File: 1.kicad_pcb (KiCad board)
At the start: 2 copper layers, 85.1 x 46.4 mm, 44 parts, among them J1 Micro_SD_Card, J10 I2C1, J11 I2C2, J12 B3..9A, J2 USB_B_Micro, J3 Conn_Power, J4 SWD, J5 Protected, J6 SPI1, J7 ADC, J8 UART1, J9 SPI2, K1 NRST, K2 WKUP, K3 KPA0, U1 STM32F103C8Tx, U2 AMS1117-3.3, Y1 8MHz, Y2 32.768k

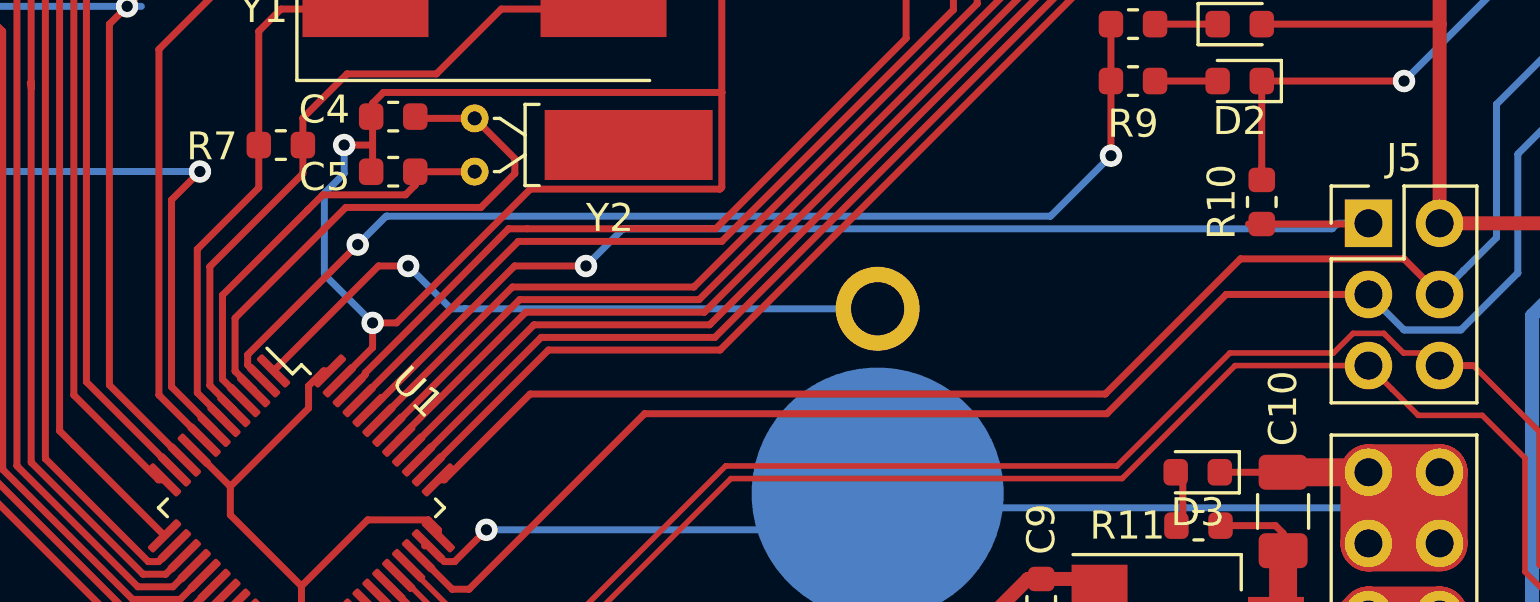
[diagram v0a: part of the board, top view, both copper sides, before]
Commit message: ops
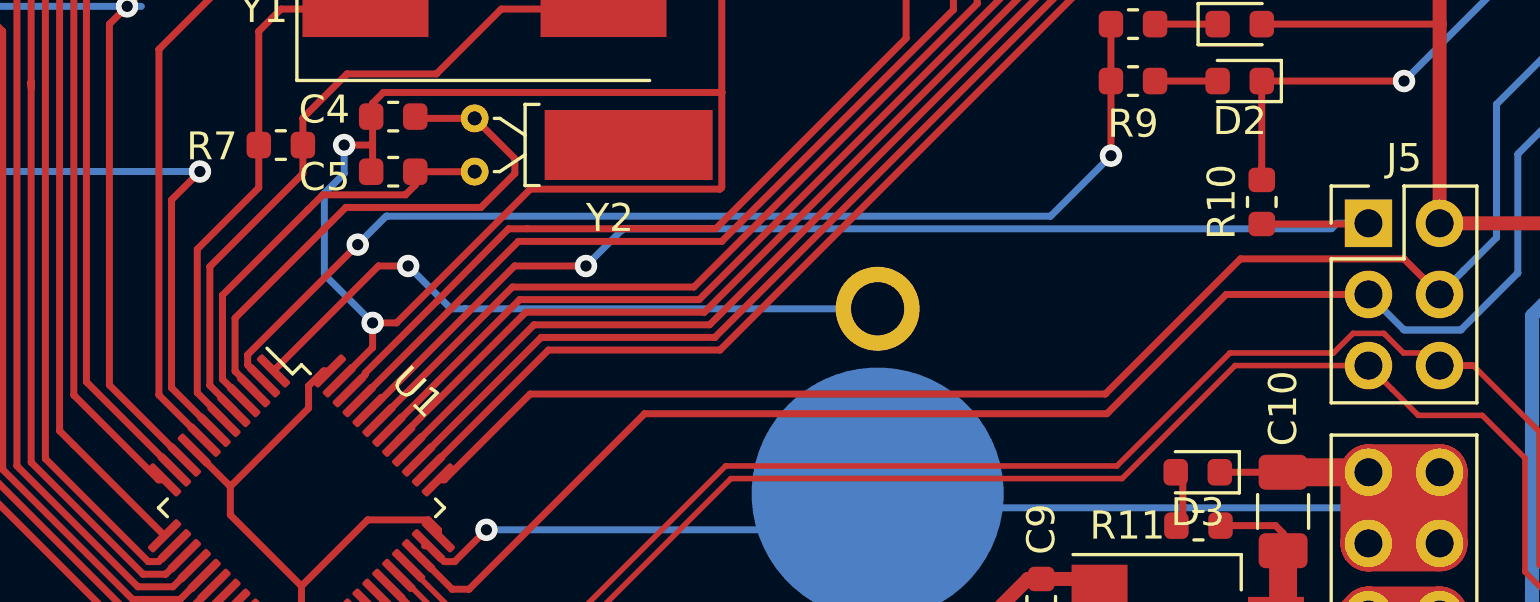
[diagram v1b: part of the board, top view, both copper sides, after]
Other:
- board text added: "3V3 5V"
- board text added: "C D I2C1"
- board text added: "I O K S SPI1"
- board text removed: ". . . . SPI1"
- board text removed: ". . I2C1"
- board text removed: "GND 3V3 5V"
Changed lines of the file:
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@@
   (general
     (thickness 1.6)
-    (drawings 43)
+    (drawings 44)
     (tracks 645)
     (zones 0)
@@
     )
   )
+  (gr_text GND (at 172.72 118.11) (layer Eco2.User)
+    (effects (font (size 1 1) (thickness 0.15)))
+  )
+  (gr_text "I  O K S\nSPI1" (at 160.274 97.79) (layer Eco1.User)
+    (effects (font (size 1.2 1.2) (thickness 0.15)))
+  )
   (gr_text "TIM1\n1  2  3" (at 144.78 126.492) (layer Eco2.User)
-    (effects (font (size 1 1) (thickness 0.15)))
+    (effects (font (size 1 1) (thickness 0.2)))
   )
   (gr_text "TIM2   3   4" (at 113.284 122.174) (layer Eco2.User)
     (effects (font (size 0.8 0.8) (thickness 0.15)))
   )
-  (gr_text ".  .  .  .\nSPI1" (at 115.824 99.314) (layer Eco1.User)
-    (effects (font (size 1.25 1.25) (thickness 0.2)))
+  (gr_text "I  O K S\nSPI1" (at 115.824 100.33) (layer Eco1.User)
+    (effects (font (size 1.05 1.05) (thickness 0.2)))
   )
   (gr_text "UART3  Tx  Rx" (at 113.284 123.444) (layer Eco1.User)
     (effects (font (size 0.8 0.8) (thickness 0.15)))
   )
-  (gr_text ".  .\nI2C1" (at 152.527 97.028) (layer Eco2.User)
+  (gr_text "C  D\nI2C1" (at 152.527 97.79) (layer Eco2.User)
     (effects (font (size 1.25 1.25) (thickness 0.2)))
   )
-  (gr_text "2  1\nTIM2" (at 146.812 90.932) (layer Eco1.User)
+  (gr_text "2  1\nTIM2" (at 147.32 91.186) (layer Eco1.User)
     (effects (font (size 0.8 0.8) (thickness 0.15)) (justify right))
   )
-  (gr_text "GND\n\n\n3V3\n\n\n5V" (at 172.847 123.19) (layer Eco2.User)
+  (gr_text "3V3\n\n\n5V" (at 172.847 125.73) (layer Eco1.User)
     (effects (font (size 1.1 1.1) (thickness 0.2)))
   )
@@
     (effects (font (size 0.8 0.8) (thickness 0.2)))
   )
-  (gr_text "2  1\nTIM3" (at 143.256 90.932) (layer Eco2.User)
+  (gr_text "2  1\nTIM3" (at 143.51 91.186) (layer Eco2.User)
     (effects (font (size 0.8 0.8) (thickness 0.15)) (justify right))
   )
@@
     (effects (font (size 0.65 0.65) (thickness 0.15)))
   )
-  (gr_text "TIM4  2  1\n4  3" (at 136.525 89.535) (layer Eco1.User)
+  (gr_text "TIM4  2  1\n4  3" (at 136.779 89.789) (layer Eco1.User)
     (effects (font (size 0.8 0.8) (thickness 0.15)) (justify left))
-  )
-  (gr_text ".  .  .  .\nSPI1" (at 160.147 97.028) (layer Eco1.User)
-    (effects (font (size 1.25 1.25) (thickness 0.2)))
   )
   (gr_text OSC (at 127 109.982) (layer Dwgs.User)
@@
     (effects (font (size 1.55 1.55) (thickness 0.25)) (justify left))
   )
-  (gr_text "Tx Rx\nUART2" (at 123.571 99.695) (layer Eco1.User)
-    (effects (font (size 1 1) (thickness 0.15)))
+  (gr_text "Tx Rx\nUART2" (at 123.698 100.33) (layer Eco1.User)
+    (effects (font (size 1.05 1.05) (thickness 0.2)))
   )
   (gr_text "A0\nA1\nA2\nA3\nA4\nA5\nA6\nA7\nB0\nB1" (at 118.237 93.98 270) (layer Dwgs.User)
     (effects (font (size 1.5 1.5) (thickness 0.3)))
   )
-  (gr_text "4  3  2  1\nTIM2" (at 126.111 96.901) (layer Eco2.User)
-    (effects (font (size 1 1) (thickness 0.15)))
-  )
-  (gr_text "4  3  2  1\nTIM3" (at 110.617 96.901) (layer Eco2.User)
-    (effects (font (size 1 1) (thickness 0.15)))
+  (gr_text "4  3  2  1\nTIM2" (at 125.984 96.901) (layer Eco2.User)
+    (effects (font (size 1.05 1.05) (thickness 0.2)))
+  )
+  (gr_text "4  3  2  1\nTIM3" (at 110.744 97.028) (layer Eco2.User)
+    (effects (font (size 1.05 1.05) (thickness 0.2)))
   )
   (segment (start 135.656008 130.192212) (end 135.443876 130.192212) (width 0.25) (layer F.Cu) (net 1))
@@
   (segment (start 125.9135 106.1015) (end 125.9135 106.1015) (width 0.25) (layer B.Cu) (net 5))
   (via (at 125.9135 106.1015) (size 0.8) (drill 0.4) (layers F.Cu B.Cu) (net 5))
-  (segment (start 124.900666 107.114334) (end 125.9135 106.1015) (width 0.25) (layer F.Cu) (net 5))
-  (segment (start 124.900666 113.788878) (end 124.900666 107.114334) (width 0.25) (layer F.Cu) (net 5))
-  (segment (start 126.419891 115.308103) (end 124.900666 113.788878) (width 0.25) (layer F.Cu) (net 5))
   (segment (start 126.419891 115.343445) (end 126.419891 115.308103) (width 0.25) (layer F.Cu) (net 5))
+  (segment (start 124.900666 113.82422) (end 126.419891 115.343445) (width 0.25) (layer F.Cu) (net 5))
+  (segment (start 124.900666 107.114334) (end 124.900666 113.82422) (width 0.25) (layer F.Cu) (net 5))
+  (segment (start 125.9135 106.1015) (end 124.900666 107.114334) (width 0.25) (layer F.Cu) (net 5))
   (segment (start 133.934717 119.469322) (end 133.970057 119.469322) (width 0.25) (layer F.Cu) (net 7))
   (segment (start 134.366 96.266) (end 137.871 96.266) (width 0.25) (layer F.Cu) (net 7))
@@
   (segment (start 163.068 109.22) (end 168.91 109.22) (width 0.25) (layer F.Cu) (net 23))
   (segment (start 167.6145 107.9755) (end 167.64 107.95) (width 0.25) (layer F.Cu) (net 24))
-  (segment (start 163.83 107.9755) (end 167.6145 107.9755) (width 0.25) (layer F.Cu) (net 24))
-  (segment (start 163.83 107.9755) (end 163.355 107.9755) (width 0.25) (layer F.Cu) (net 24))
   (segment (start 131.988342 114.636338) (end 137.15068 109.474) (width 0.25) (layer F.Cu) (net 24))
   (segment (start 131.953002 114.636338) (end 131.988342 114.636338) (width 0.25) (layer F.Cu) (net 24))
@@
   (segment (start 139.7 109.474) (end 139.7 109.474) (width 0.25) (layer F.Cu) (net 24))
   (via (at 139.7 109.474) (size 0.8) (drill 0.4) (layers F.Cu B.Cu) (net 24))
-  (segment (start 166.54 107.95) (end 167.64 107.95) (width 0.25) (layer B.Cu) (net 24))
-  (segment (start 166.34399 108.14601) (end 166.54 107.95) (width 0.25) (layer B.Cu) (net 24))
-  (segment (start 141.02799 108.14601) (end 166.34399 108.14601) (width 0.25) (layer B.Cu) (net 24))
-  (segment (start 139.7 109.474) (end 141.02799 108.14601) (width 0.25) (layer B.Cu) (net 24))
+  (segment (start 163.83 107.9755) (end 167.6145 107.9755) (width 0.25) (layer F.Cu) (net 24))
+  (segment (start 140.97 108.204) (end 139.7 109.474) (width 0.25) (layer B.Cu) (net 24))
+  (segment (start 141.02799 108.14601) (end 140.97 108.204) (width 0.25) (layer B.Cu) (net 24))
+  (segment (start 166.31201 108.14601) (end 141.02799 108.14601) (width 0.25) (layer B.Cu) (net 24))
+  (segment (start 166.50802 107.95) (end 166.31201 108.14601) (width 0.25) (layer B.Cu) (net 24))
+  (segment (start 167.64 107.95) (end 166.50802 107.95) (width 0.25) (layer B.Cu) (net 24))
   (via (at 158.4452 105.537) (size 0.8) (drill 0.4) (layers F.Cu B.Cu) (net 25))
   (segment (start 158.445 100.838) (end 158.445 102.87) (width 0.25) (layer F.Cu) (net 25))
   (segment (start 158.445 105.5368) (end 158.4452 105.537) (width 0.25) (layer F.Cu) (net 25))
   (segment (start 158.445 102.87) (end 158.445 105.5368) (width 0.25) (layer F.Cu) (net 25))
-  (segment (start 158.4452 105.537) (end 156.2862 107.696) (width 0.25) (layer B.Cu) (net 25))
   (segment (start 127.619711 113.007731) (end 128.187658 113.575678) (width 0.25) (layer F.Cu) (net 25))
   (segment (start 127.619711 112.641007) (end 127.619711 113.007731) (width 0.25) (layer F.Cu) (net 25))
@@
   (segment (start 131.548718 108.712) (end 131.548718 108.712) (width 0.25) (layer F.Cu) (net 25))
   (via (at 131.548718 108.712) (size 0.8) (drill 0.4) (layers F.Cu B.Cu) (net 25))
+  (segment (start 131.548718 108.712) (end 132.564718 107.696) (width 0.25) (layer B.Cu) (net 25))
+  (segment (start 158.4452 105.537) (end 156.2862 107.696) (width 0.25) (layer B.Cu) (net 25))
   (segment (start 132.564718 107.696) (end 132.588 107.696) (width 0.25) (layer B.Cu) (net 25))
-  (segment (start 131.548718 108.712) (end 132.564718 107.696) (width 0.25) (layer B.Cu) (net 25))
   (segment (start 156.2862 107.696) (end 132.588 107.696) (width 0.25) (layer B.Cu) (net 25))
   (segment (start 119.888 91.44) (end 122.428 88.9) (width 0.25) (layer F.Cu) (net 26))
